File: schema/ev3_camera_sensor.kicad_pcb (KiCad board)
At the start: 2 copper layers, 39.4 x 64.8 mm, 14 parts

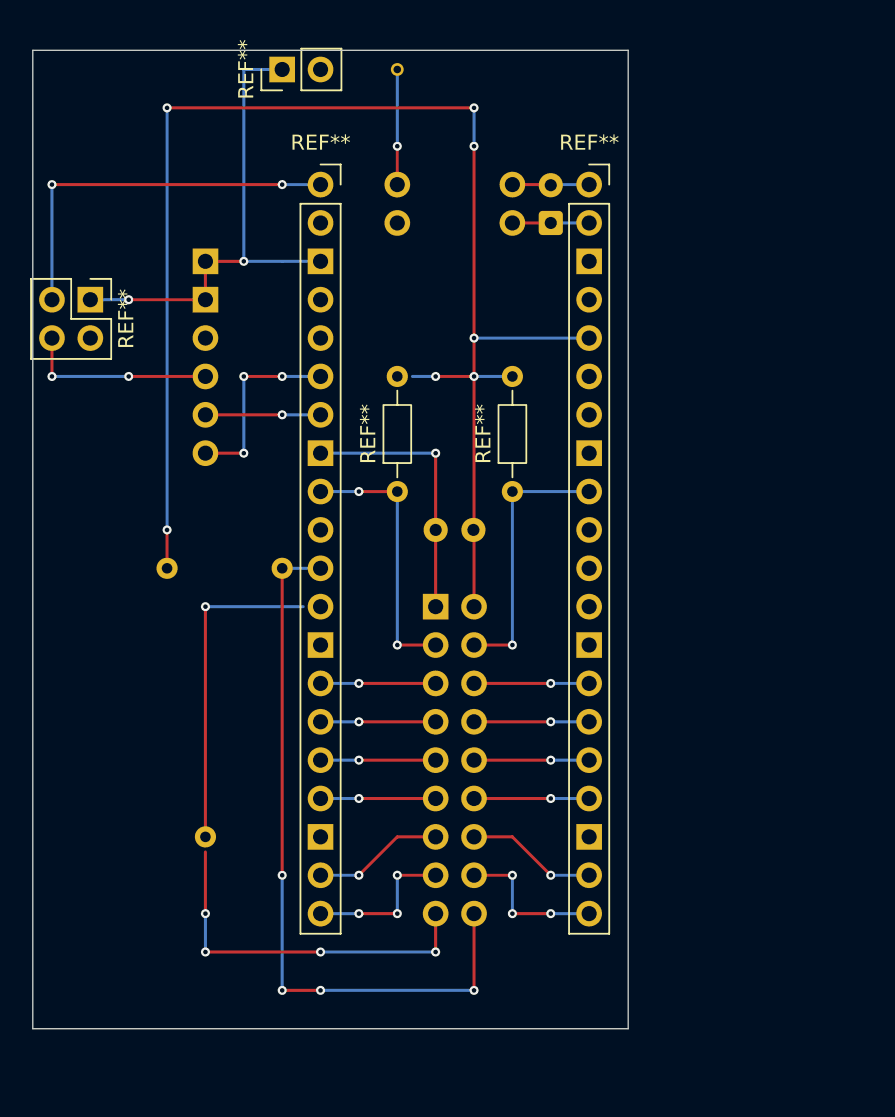
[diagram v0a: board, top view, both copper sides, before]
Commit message: update pcb
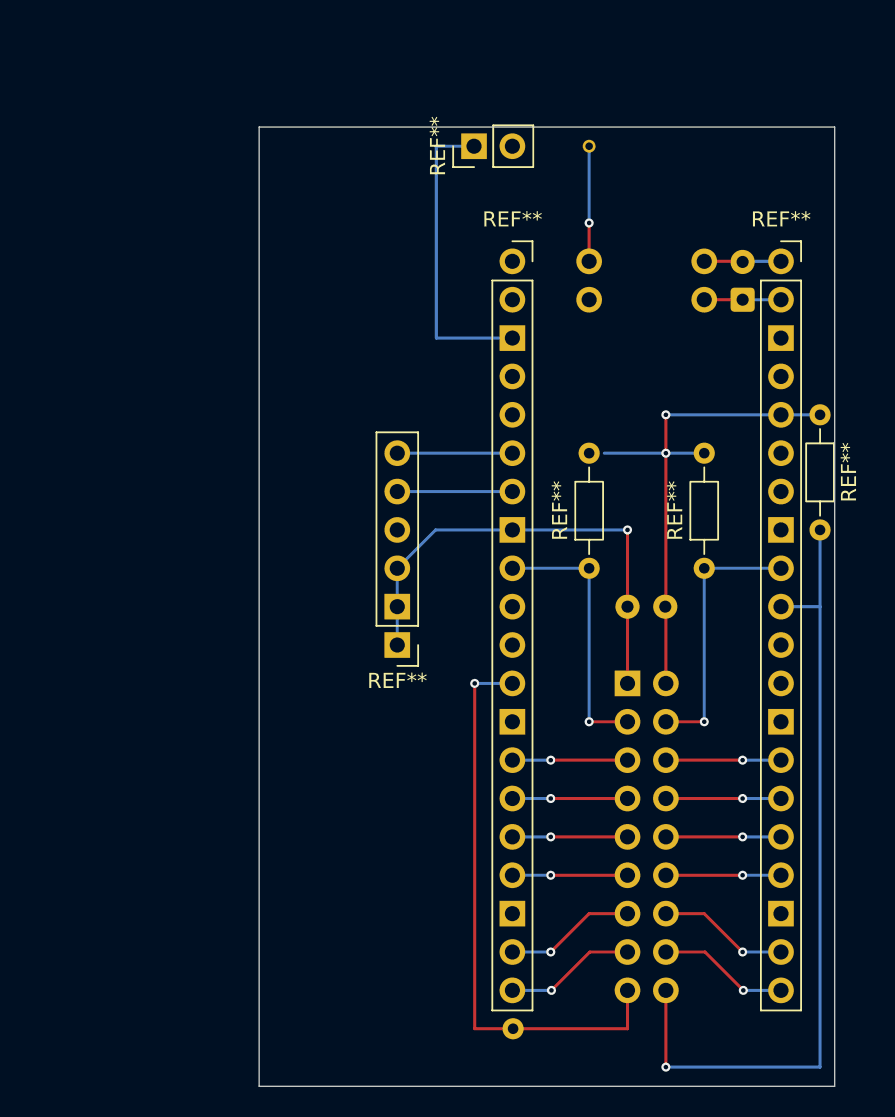
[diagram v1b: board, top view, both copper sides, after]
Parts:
- removed the REF** at (161.3, 73.7)
- removed the REF** at (156.2, 73.7)
- removed the REF** at (128.3, 81.3)
- removed the REF** at (141.0, 66.0)
- removed the REF** at (148.6, 94.0)
- removed the REF** at (143.5, 73.7)
- removed the REF** at (156.2, 94.0)
- removed the REF** at (135.9, 116.8)
- removed the REF** at (133.3, 99.1)
- added REF**: PinSocket_1x20_P2.54mm_Vertical, Connector_PinSocket_2.54mm:PinSocket_1x20_P2.54mm_Vertical, F.Cu at (174.0, 78.7)
- added REF**: PinHeader_1x02_P2.54mm_Vertical, Connector_PinHeader_2.54mm:PinHeader_1x02_P2.54mm_Vertical, B.Cu at (168.9, 78.7)
- added REF**: R_Axial_DIN0204_L3.6mm_D1.6mm_P7.62mm_Horizontal, Resistor_THT:R_Axial_DIN0204_L3.6mm_D1.6mm_P7.62mm_Horizontal, F.Cu at (176.6, 88.9)
- added REF**: R_Axial_DIN0204_L3.6mm_D1.6mm_P7.62mm_Horizontal, Resistor_THT:R_Axial_DIN0204_L3.6mm_D1.6mm_P7.62mm_Horizontal, F.Cu at (161.3, 99.1)
- added REF**: PinHeader_1x02_P2.54mm_Vertical, Connector_PinHeader_2.54mm:PinHeader_1x02_P2.54mm_Vertical, F.Cu at (153.7, 71.1)
- added REF**: PinSocket_1x20_P2.54mm_Vertical, Connector_PinSocket_2.54mm:PinSocket_1x20_P2.54mm_Vertical, F.Cu at (156.2, 78.7)
- added REF**: R_Axial_DIN0204_L3.6mm_D1.6mm_P7.62mm_Horizontal, Resistor_THT:R_Axial_DIN0204_L3.6mm_D1.6mm_P7.62mm_Horizontal, F.Cu at (168.9, 99.1)
- added REF**: R_Axial_DIN0204_L3.6mm_D1.6mm_P7.62mm_Horizontal, Resistor_THT:R_Axial_DIN0204_L3.6mm_D1.6mm_P7.62mm_Horizontal, B.Cu at (156.3, 121.9)
- REF**: moved to F.Cu
- moved REF** 29.9 mm to (148.6, 105.0)
- moved REF** 13.7 mm to (163.8, 106.7)
- moved REF** 13.7 mm to (166.3, 101.6)
- moved REF** 13.7 mm to (171.4, 81.3)
- moved REF** 13.7 mm to (161.3, 71.1)
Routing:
- net (no net): track 453.6 -> 342.1 mm, vias 52 -> 24
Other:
- board size 39.4 x 64.8 mm -> 38.1 x 63.5 mm
